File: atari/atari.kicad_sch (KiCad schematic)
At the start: 2 parts, among them J5 ADAPTER, J6 ATARI

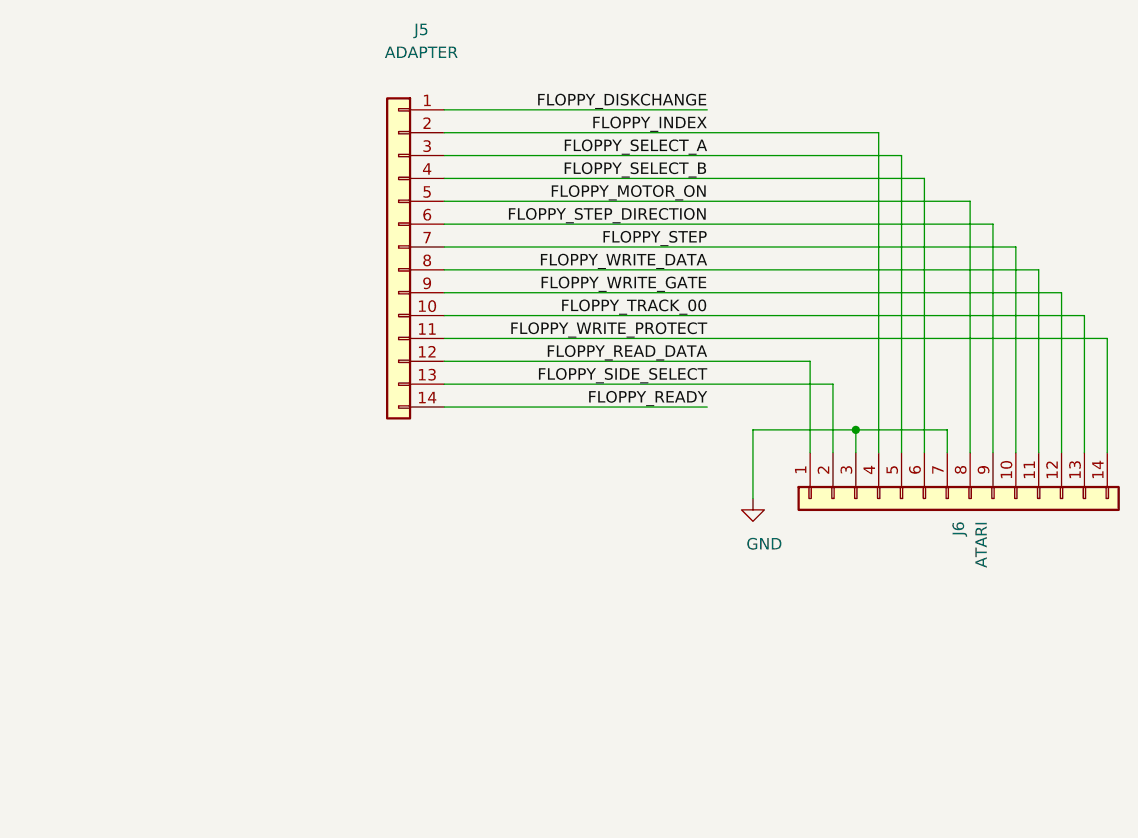
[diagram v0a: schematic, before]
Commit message: a
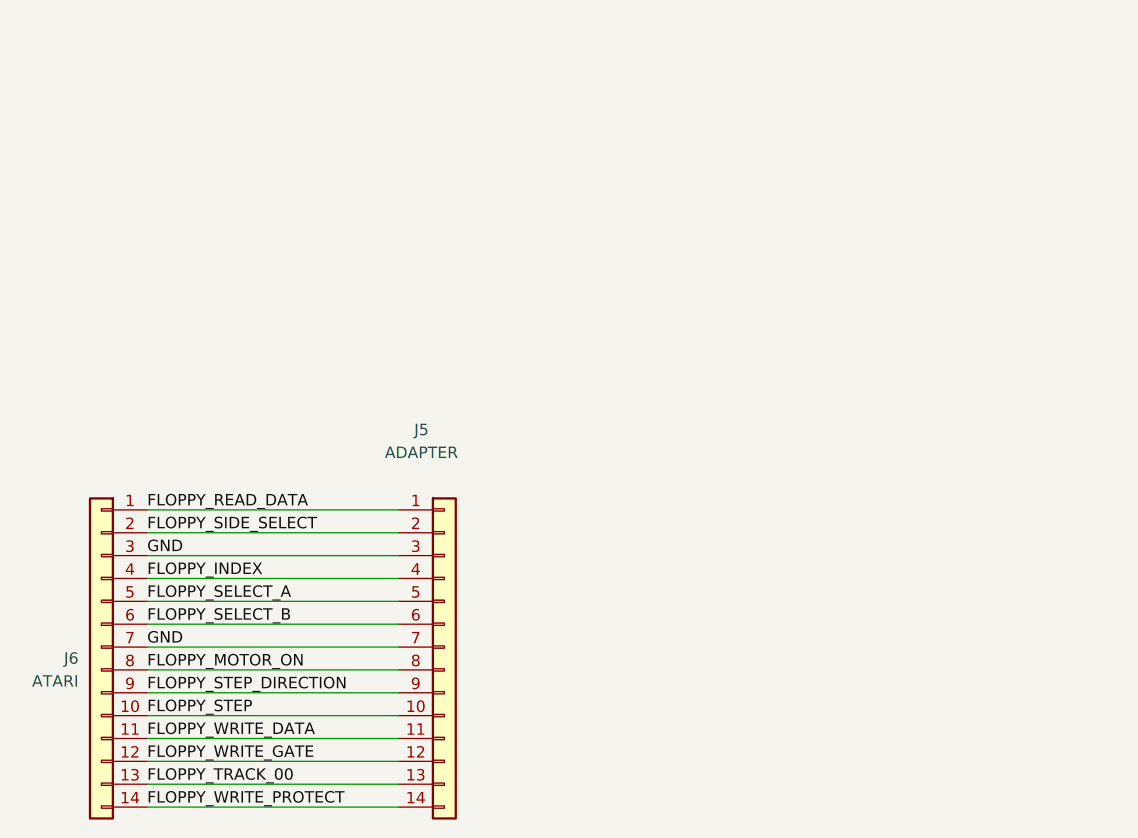
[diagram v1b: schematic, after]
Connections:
- net FLOPPY_DISKCHANGE is gone; now on net FLOPPY_READ_DATA: J5.1 (Pin_1)
- net FLOPPY_READY is gone; now on net FLOPPY_WRITE_PROTECT: J5.14 (Pin_14)
- net FLOPPY_INDEX: now also J5.4 (Pin_4); no longer J5.2 (Pin_2)
- net FLOPPY_MOTOR_ON: now also J5.8 (Pin_8); no longer J5.5 (Pin_5)
- net FLOPPY_READ_DATA: no longer J5.12 (Pin_12)
- net FLOPPY_SELECT_A: now also J5.5 (Pin_5); no longer J5.3 (Pin_3)
- net FLOPPY_SELECT_B: now also J5.6 (Pin_6); no longer J5.4 (Pin_4)
- net FLOPPY_SIDE_SELECT: now also J5.2 (Pin_2); no longer J5.13 (Pin_13)
- net FLOPPY_STEP: now also J5.10 (Pin_10); no longer J5.7 (Pin_7)
- net FLOPPY_STEP_DIRECTION: now also J5.9 (Pin_9); no longer J5.6 (Pin_6)
- net FLOPPY_TRACK_00: now also J5.13 (Pin_13); no longer J5.10 (Pin_10)
- net FLOPPY_WRITE_DATA: now also J5.11 (Pin_11); no longer J5.8 (Pin_8)
- net FLOPPY_WRITE_GATE: now also J5.12 (Pin_12); no longer J5.9 (Pin_9)
- net FLOPPY_WRITE_PROTECT: no longer J5.11 (Pin_11)
- net GND: now also J5.3 (Pin_3), J5.7 (Pin_7)
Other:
- moved on the sheet: J5, J6
